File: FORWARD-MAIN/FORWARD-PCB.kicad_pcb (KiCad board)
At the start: 4 copper layers, 98 x 98 mm, 50 parts, among them J1 USB_B_Micro, J2 Conn_01x15_Socket, J3 Conn_01x02_Pin, J4 Conn_01x08_Socket, J5 Conn_01x03_Socket, J6 Conn_01x02_Pin, Q1 SS8050-G, Q2 SS8050-G, U2 CP2102N-Axx-xQFN28, U5 ESP32-WROOM-32D

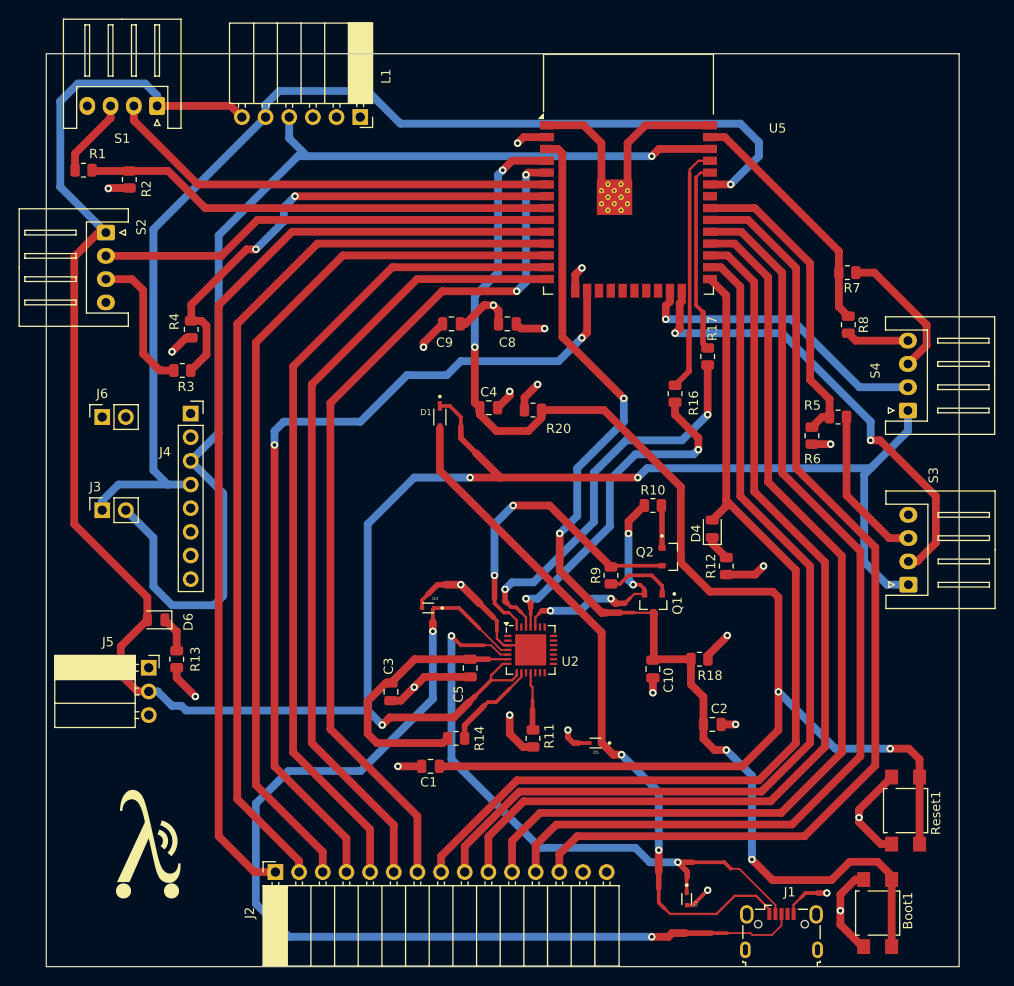
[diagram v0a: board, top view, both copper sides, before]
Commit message: re-routing rev 2.0
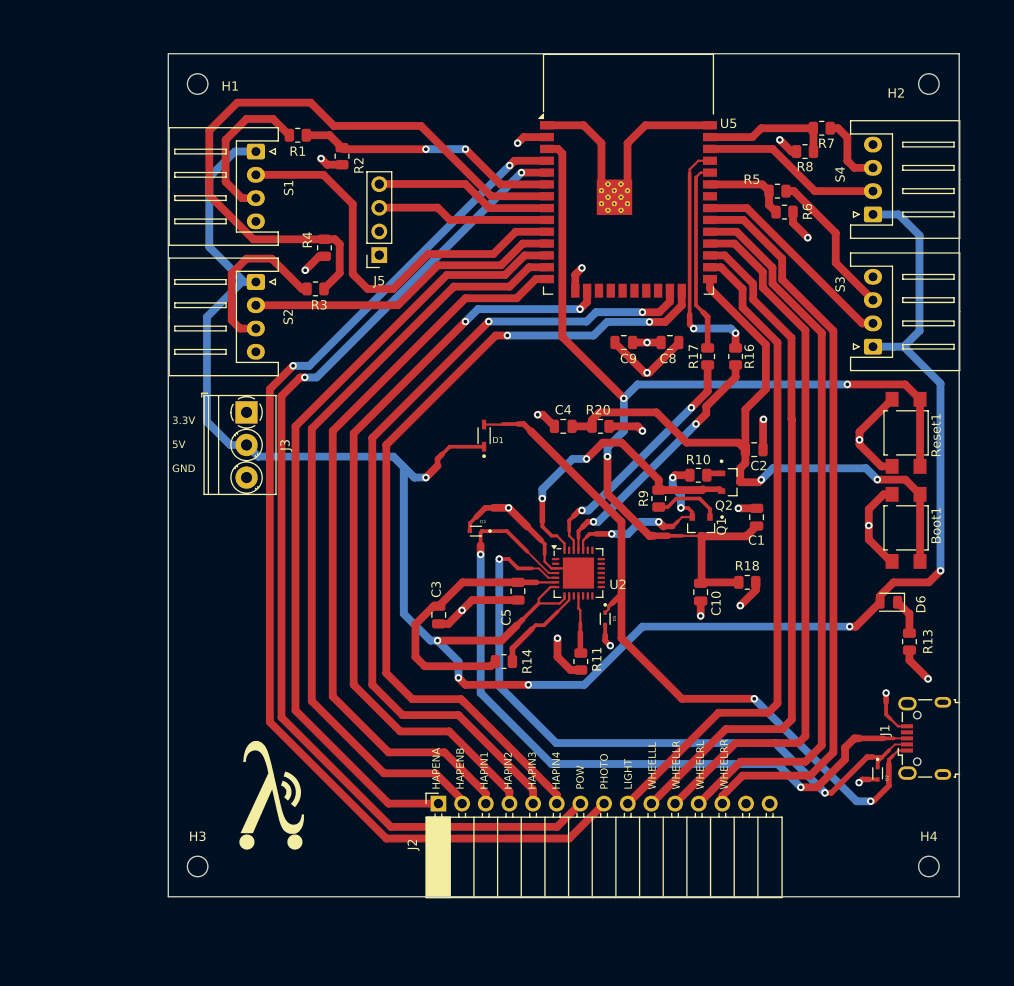
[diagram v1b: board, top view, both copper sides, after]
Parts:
- removed D4: LED, LED_SMD:LED_0805_2012Metric
- removed J4: Conn_01x08_Socket, Connector_PinSocket_2.54mm:PinSocket_1x08_P2.54mm_Vertical
- removed J6: Conn_01x02_Pin, Connector_PinSocket_2.54mm:PinSocket_1x02_P2.54mm_Vertical
- removed L1: Conn_01x06_Socket, Connector_PinSocket_2.54mm:PinSocket_1x06_P2.54mm_Horizontal
- removed R12: 1k, Resistor_SMD:R_0805_2012Metric
- added H1: MountingHole, MountingHole:MountingHole_2.2mm_M2, F.Cu at (117.8, 51.8)
- added H2: MountingHole, MountingHole:MountingHole_2.2mm_M2, F.Cu at (196.2, 51.8)
- added H3: MountingHole, MountingHole:MountingHole_2.2mm_M2, F.Cu at (117.8, 135.8)
- added H4: MountingHole, MountingHole:MountingHole_2.2mm_M2, F.Cu at (196.2, 135.8)
- J3: value Conn_01x02_Pin -> Screw_Terminal_01x03; footprint Connector_PinSocket_2.54mm:PinSocket_1x02_P2.54mm_Vertical -> TerminalBlock_Phoenix:TerminalBlock_Phoenix_PT-1,5-3-3.5-H_1x03_P3.50mm_Horizontal
- J5: value Conn_01x03_Socket -> Conn_01x04_Socket; footprint Connector_PinSocket_2.54mm:PinSocket_1x03_P2.54mm_Horizontal -> Connector_PinSocket_2.54mm:PinSocket_1x04_P2.54mm_Vertical
- moved D6 78.7 mm to (191.9, 107.4)
- moved R13 78.7 mm to (194.2, 111.6)
- moved J5 50.7 mm to (137.2, 70.1), turned to 180 degrees
- moved C1 44.1 mm to (177.8, 98.2), turned to 90 degrees
- moved Boot1 41.5 mm to (193.8, 99.4)
- moved Reset1 40.6 mm to (193.8, 89.2)
- moved C2 29.8 mm to (177.5, 91.0)
- moved S3 25.8 mm to (190.2, 80.0)
- moved J1 25.8 mm to (195.8, 122.0), turned to 90 degrees
- moved R5 25.1 mm to (180.0, 63.2)
- moved D2 24.5 mm to (190.8, 125.8)
- moved R6 24.2 mm to (180.8, 65.5), turned to 0 degrees
- moved R1 23.3 mm to (128.5, 57.2)
- moved R2 23.0 mm to (133.2, 59.5)
- moved S4 21.4 mm to (190.2, 65.8)
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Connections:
- Boot1 pad 2: /EN -> /BOOT
- C1 pad 1: /IO0 -> /EN
- C2 pad 1: /EN -> /BOOT
- C4 pad 1: /IO0 -> /BOOT
- J2 pad 1: /Haptics-IN1 -> /Haptics-ENA_PWM
- J2 pad 2: /Haptics-IN2 -> /Haptics-ENB_PWM
- J2 pad 3: /Haptics-IN3 -> /Haptics-IN1
- J2 pad 4: /Haptics-IN4 -> /Haptics-IN2
- J2 pad 5: /Haptics-ENA_PWM -> /Haptics-IN3
- J2 pad 6: /Haptics-ENB_PWM -> /Haptics-IN4
- J3 pad 1: /SDA -> +3.3V
- J3 pad 2: /SCL -> +5V
- J5 pad 2: +5V -> GND
- J5 pad 3: GND -> /SCL
- Q2 pad 3: /IO0 -> /BOOT
- R20 pad 2: /IO0 -> /BOOT
- Reset1 pad 2: /IO0 -> /EN
- U5 pad 10: /Haptics-IN1 -> /TRIG_1
- U5 pad 11: /Haptics-IN2 -> /TRIG_2
- U5 pad 12: /Haptics-IN3 -> /Haptics-ENA_PWM
- U5 pad 13: /Haptics-ENA_PWM -> /Haptics-ENB_PWM
- U5 pad 14: /Haptics-ENB_PWM -> /Haptics-IN1
- U5 pad 16: /Haptics-IN4 -> /Haptics-IN2
- U5 pad 23: /TRIG_4 -> /Haptics-IN3
- U5 pad 24: /TRIG_3 -> /Haptics-IN4
- U5 pad 25: /PHOTO-IO2-24 -> /BOOT
- U5 pad 31: /ECHO_3 -> /TRIG_3
- U5 pad 33: /SDA -> /ECHO_3
- U5 pad 36: /SCL -> /TRIG_4
- U5 pad 4: /IO0 -> /PHOTO-IO2-24
- U5 pad 6: /TRIG_1 -> /ECHO_1
- U5 pad 8: /ECHO_1 -> /SDA
- U5 pad 9: /TRIG_2 -> /SCL
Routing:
- net /IO0: track 159.7 -> 0.00 mm, vias 4 -> 0
- net /SCL: track 121.2 -> 18.6 mm, vias 1 -> 0
- net /SDA: track 121.5 -> 19.1 mm, vias 1 -> 0
- net /BOOT: track 0.00 -> 75.0 mm, vias 0 -> 2
- net /USB_DP: track 113.8 -> 80.2 mm
- net +5V: track 254.3 -> 221.5 mm, vias 3 -> 6
- net /Wheel_L_LPWM: track 102.9 -> 73.2 mm
- net /LIGHT-IO4-26: track 100.7 -> 71.1 mm
- net /Wheel_R_LPWM: track 106.7 -> 77.6 mm
- net /Wheel_L_RPWM: track 104.7 -> 75.7 mm
- net /Wheel_R_RPWM: track 108.1 -> 79.4 mm
- net /TRIG_3: track 50.1 -> 22.6 mm, vias 2 -> 0
- net /ECHO_3: track 32.9 -> 9.20 mm
- net /Haptics-IN1: track 103.2 -> 80.1 mm
- net /ECHO_1: track 50.5 -> 28.0 mm, vias 0 -> 2
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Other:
- board size 98 x 98 mm -> 84.9 x 90.5 mm
- board text added: "3.3V 5V GND"
- board text added: "HAPENA HAPENB HAPIN1 HAPIN2 HAPIN3 HAPIN4 POW PHOTO LIGHT WHEELLL WHEELLR WHEELRL WHEELRR"
